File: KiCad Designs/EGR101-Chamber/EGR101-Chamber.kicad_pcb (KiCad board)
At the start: 2 copper layers, 25.5 x 58.5 mm, 20 parts, among them J1 GX12 Interface, J2 Power Supply, J3 Pi Zero, J4 Potentiometer, J5 Switch 1, J6 Switch 2, J7 PWM Out, U1 MAX3485, U2 LMR33620BDDA

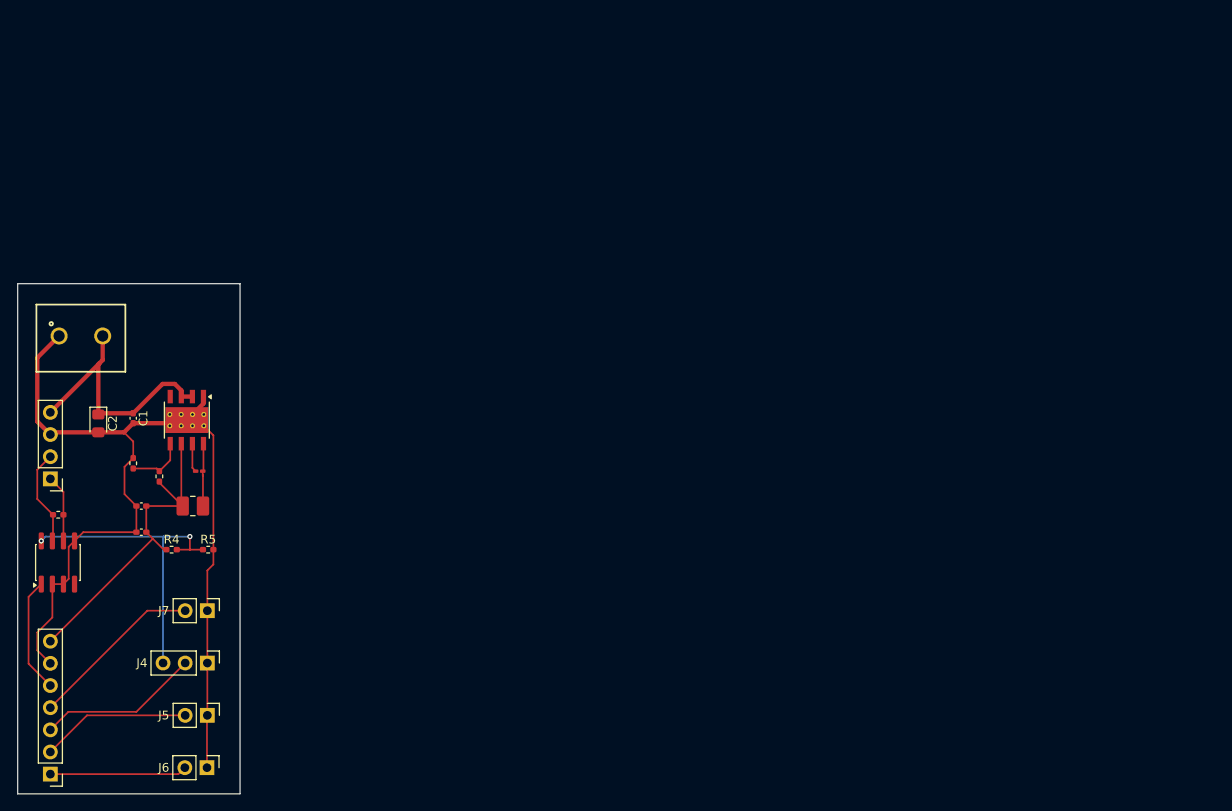
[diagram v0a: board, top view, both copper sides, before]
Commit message: Chamber PCB Finished
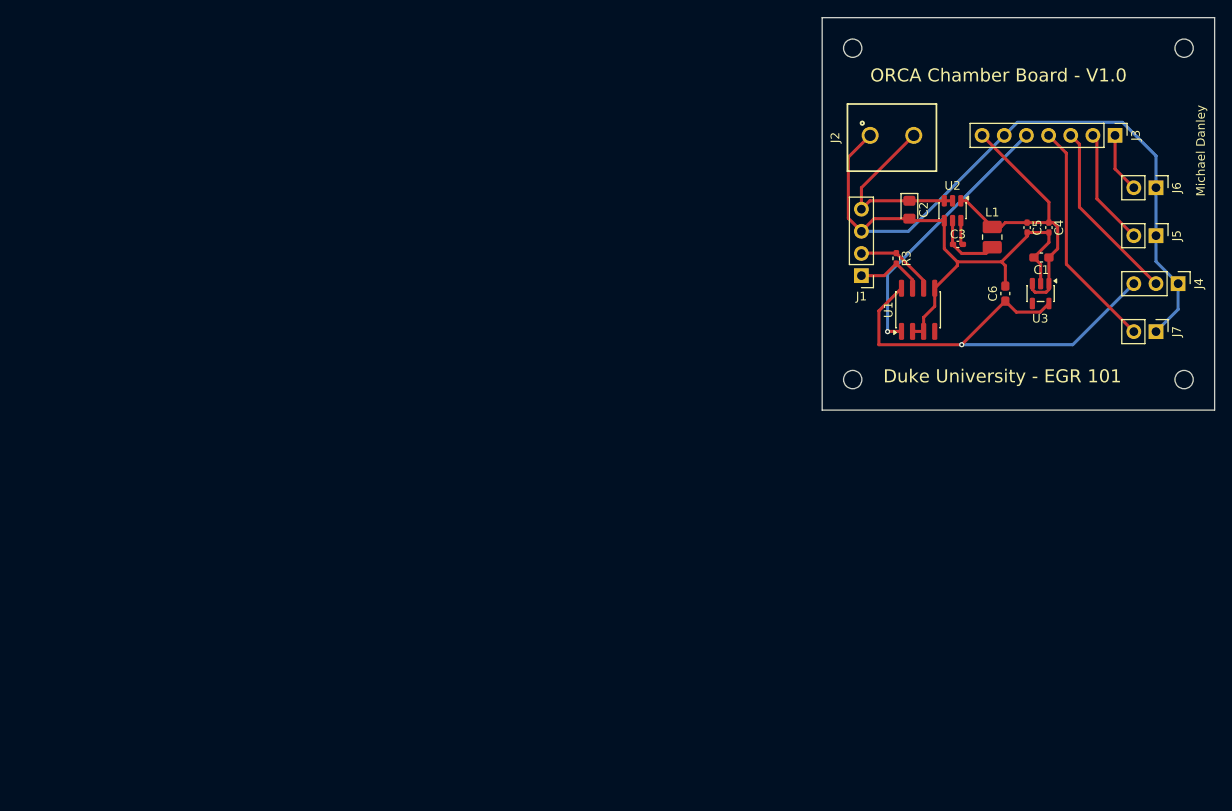
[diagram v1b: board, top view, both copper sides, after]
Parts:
- removed R1: 100 kΩ, Resistor_SMD:R_0402_1005Metric_Pad0.72x0.64mm_HandSolder
- removed R2: 24.9 kΩ, Resistor_SMD:R_0402_1005Metric_Pad0.72x0.64mm_HandSolder
- removed R4: 1 kΩ, Resistor_SMD:R_0402_1005Metric_Pad0.72x0.64mm_HandSolder
- removed R5: 2 kΩ, Resistor_SMD:R_0402_1005Metric_Pad0.72x0.64mm_HandSolder
- added C6: 1 uF, Capacitor_SMD:C_0603_1608Metric_Pad1.08x0.95mm_HandSolder, F.Cu at (198.5, 57.6)
- added H1: MountingHole, MountingHole:MountingHole_2.1mm, F.Cu at (219.0, 29.5)
- added H2: MountingHole, MountingHole:MountingHole_2.1mm, F.Cu at (181.0, 29.5)
- added H3: MountingHole, MountingHole:MountingHole_2.1mm, F.Cu at (219.0, 67.5)
- added H4: MountingHole, MountingHole:MountingHole_2.1mm, F.Cu at (181.0, 67.5)
- added U3: AP2112K-3.3, Package_TO_SOT_SMD:SOT-23-5, F.Cu at (202.6, 57.6)
- C1: value 220 nF -> 1 uF; footprint Capacitor_SMD:C_0402_1005Metric_Pad0.74x0.62mm_HandSolder -> Capacitor_SMD:C_0603_1608Metric_Pad1.08x0.95mm_HandSolder
- C3: value 0.1 uf -> 100 nF; footprint Capacitor_SMD:C_0201_0603Metric_Pad0.64x0.40mm_HandSolder -> Capacitor_SMD:C_0402_1005Metric_Pad0.74x0.62mm_HandSolder
- J1: value GX12 Interface -> External Connection
- L1: value 2.2 uH -> 4.7 uH
- U2: value LMR33620BDDA -> AP63205WU; footprint Package_SO:Texas_HSOP-8-1EP_3.9x4.9mm_P1.27mm_ThermalVias -> Package_TO_SOT_SMD:TSOT-23-6
- moved J3 142.4 mm to (211.1, 39.5), turned to -90 degrees
- moved J6 127.5 mm to (215.8, 45.5)
- moved J5 121.9 mm to (215.8, 51.0)
- moved J4 119.5 mm to (218.3, 56.5)
- moved J7 113.4 mm to (215.8, 62.0)
- moved C4 108.9 mm to (203.5, 50.1), turned to -90 degrees
- moved C5 107.4 mm to (201.0, 50.1), turned to -90 degrees
- moved C1 105.8 mm to (202.6, 53.5), turned to 180 degrees
- moved U1 102.8 mm to (188.5, 59.5)
- moved R3 100.5 mm to (186.0, 53.6), turned to -90 degrees
- moved L1 96.7 mm to (197.0, 51.2), turned to 90 degrees
- moved C2 96.2 mm to (187.5, 48.0)
- moved J1 95.9 mm to (182.0, 55.6)
- moved J2 95.8 mm to (185.5, 39.5)
- moved U2 91.0 mm to (192.4, 48.1)
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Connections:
- C1 pad 1: Net-(J1-Pin_4) -> Net-(J3-Pin_7)
- C3 pad 1: Net-(U2-BOOT) -> Net-(U2-SW)
- C3 pad 2: Net-(U2-SW) -> Net-(U2-BST)
- R3 pad 1: Net-(J1-Pin_1) -> Net-(J1-Pin_2)
- R3 pad 2: Net-(J1-Pin_2) -> Net-(J1-Pin_1)
- U1 pad 6: Net-(J1-Pin_1) -> Net-(J1-Pin_2)
- U1 pad 7: Net-(J1-Pin_2) -> Net-(J1-Pin_1)
- U2 pad 1: Net-(J1-Pin_3) -> Net-(J3-Pin_7)
- U2 pad 4: unconnected-(U2-PG-Pad4) -> Net-(J1-Pin_3)
- U2 pad 5: Net-(U2-FB) -> Net-(U2-SW)
- U2 pad 6: Net-(J3-Pin_7) -> Net-(U2-BST)
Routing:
- net Net-(J3-Pin_5): track 13.3 -> 30.7 mm, vias 0 -> 1
- net Net-(J4-Pin_3): track 36.3 -> 52.7 mm, vias 2 -> 1
- net Net-(J1-Pin_3): track 112.5 -> 123.9 mm
- net Net-(J3-Pin_1): track 15.7 -> 6.89 mm
- net Net-(J1-Pin_4): track 30.6 -> 21.8 mm
- net Net-(U2-FB): track 6.79 -> 0.00 mm
- net Net-(J3-Pin_4): track 20.1 -> 26.5 mm
- net Net-(J3-Pin_2): track 17.2 -> 13.4 mm
- net Net-(U2-BOOT): track 3.31 -> 0.00 mm
- net Net-(U2-BST): track 0.00 -> 2.76 mm
- net Net-(J3-Pin_3): track 18.6 -> 21.0 mm
- net Net-(J1-Pin_2): track 11.1 -> 9.34 mm
- net Net-(J3-Pin_7): track 38.1 -> 36.3 mm
- net Net-(U2-SW): track 7.19 -> 7.99 mm
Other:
- board size 25.5 x 58.5 mm -> 45 x 45 mm
- board text added: "Duke University - EGR 101"
- board text added: "Michael Danley"
- board text added: "ORCA Chamber Board - V1.0"
